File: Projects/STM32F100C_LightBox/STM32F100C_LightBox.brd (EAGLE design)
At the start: 50 x 50 mm, 1 part

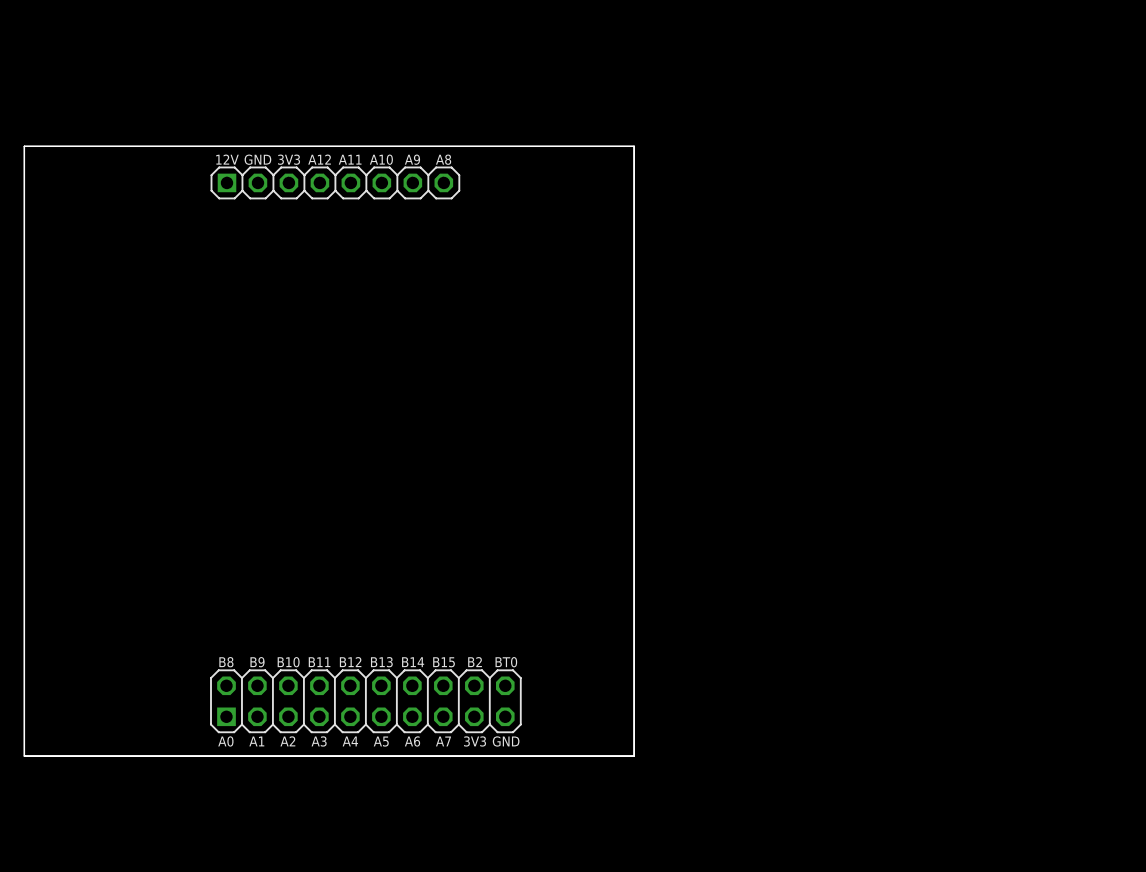
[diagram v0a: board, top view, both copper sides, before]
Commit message: LiteBox Project started...
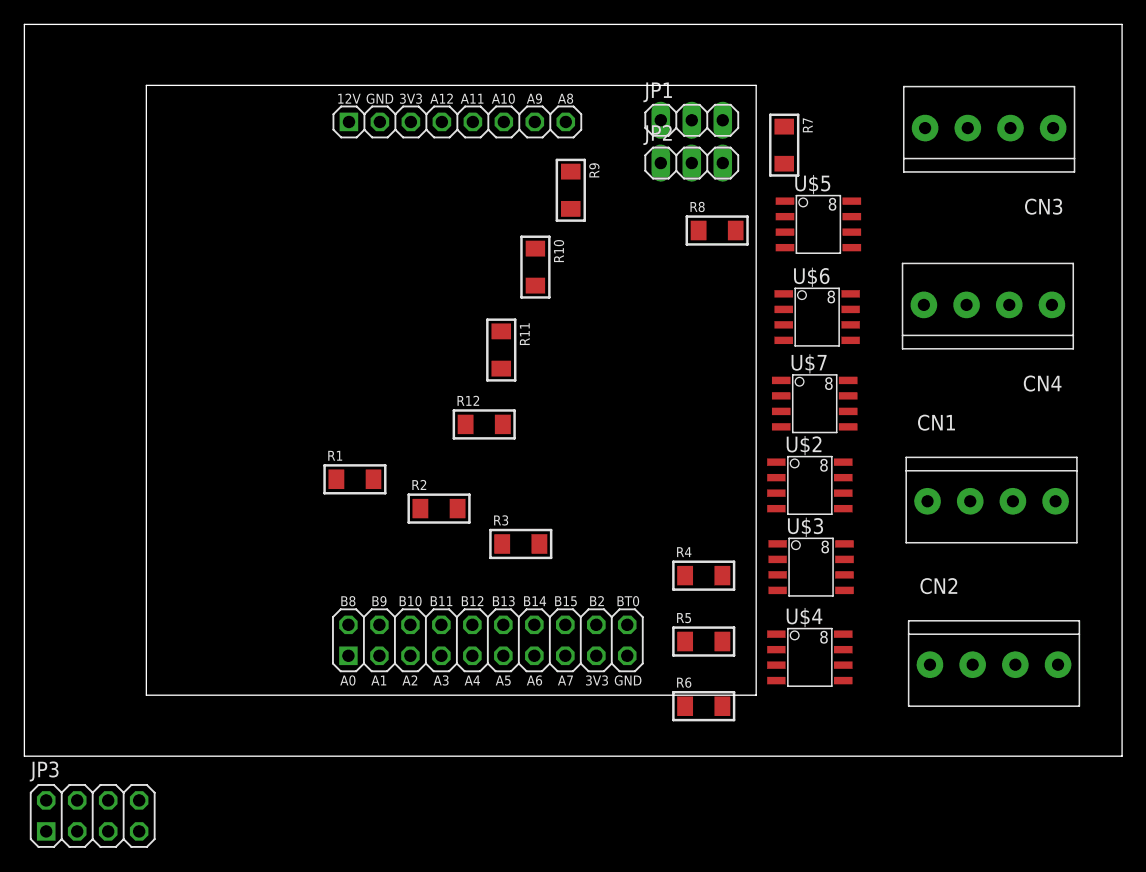
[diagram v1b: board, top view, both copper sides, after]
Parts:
- added CN1, CN2, CN3, CN4: 1X4-3.5MM, adafruit:1X04-3.5MM
- added JP1: DHT11, pinhead-2:1X03
- added JP2: DS1820, pinhead-2:1X03
- added JP3: (no value), pinhead-2:2X04
- added R1, R10, R11, R12, R2, R3, R4, R5, R6, R7, R8, R9: 150, rc-master-smd:R1206
- added U$2, U$3, U$4, U$5, U$6, U$7: IRF7313, my-library:SO-8
- moved U$1 11.2 mm to (10.0, 5.00)
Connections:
- new net GND: U$2.1, U$2.3, U$3.1, U$3.3, U$4.1, U$4.3, U$5.1, U$5.3, U$6.1, U$6.3, U$7.1, U$7.3
- new net N$1: CN1.2, U$2.7, U$2.8
- new net N$10: R4.2, U$3.4
- new net N$11: R5.2, U$4.2
- new net N$12: CN3.2, U$5.7, U$5.8
- new net N$13: CN3.3, U$5.5, U$5.6
- new net N$14: CN3.4, U$6.7, U$6.8
- new net N$15: CN4.2, U$6.5, U$6.6
- new net N$16: CN4.3, U$7.7, U$7.8
- new net N$17: CN4.4, U$7.5, U$7.6
- new net N$18: R7.2, U$5.2
- new net N$19: R8.2, U$5.4
- new net N$2: CN1.3, U$2.5, U$2.6
- new net N$20: R9.2, U$6.2
- new net N$21: R10.2, U$6.4
- new net N$22: R11.2, U$7.2
- new net N$23: R6.2, U$4.4
- new net N$24: R12.2, U$7.4
- new net N$3: CN1.4, U$3.7, U$3.8
- new net N$4: CN2.2, U$3.5, U$3.6
- new net N$5: CN2.3, U$4.7, U$4.8
- new net N$6: CN2.4, U$4.5, U$4.6
- new net N$7: R1.2, U$2.2
- new net N$8: R2.2, U$2.4
- new net N$9: R3.2, U$3.2
- new net T1C1: R9.1, U$1.PA8
- new net T1C2: R10.1, U$1.PA9
- new net T1C3: R11.1, U$1.PA10
- new net T1C4: R12.1, U$1.PA11
- new net T2C1: R1.1, U$1.PA0
- new net T2C2: R2.1, U$1.PA1
- new net T2C3: R3.1, U$1.PA2
- new net T2C4: R4.1, U$1.PA3
- new net T3C1: R5.1, U$1.PA6
- new net T3C2: R6.1, U$1.PA7
- new net T3C3: JP1.2, R7.1
- new net T3C4: JP2.2, R8.1
- net +12V: now also CN1.1, CN2.1, CN3.1, CN4.1
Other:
- board size 50 x 50 mm -> 90 x 60 mm
